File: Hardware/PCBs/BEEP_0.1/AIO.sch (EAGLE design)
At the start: 79 parts, among them IC1 ULN2803ASOP18, IC2 ULN2803ASOP18, IC3 74HC238SSOP, IC4 74HC238SSOP, IC5 TS34119SMD, U2 TB6612FNG, U3 ATXMEGA64D3-AU, X10 MICROMATCH-10, X3 MICROMATCH-8, X4 MICROMATCH-8, X5 MICROMATCH-8, X8 MICROMATCH-8, X9 MICROMATCH-4

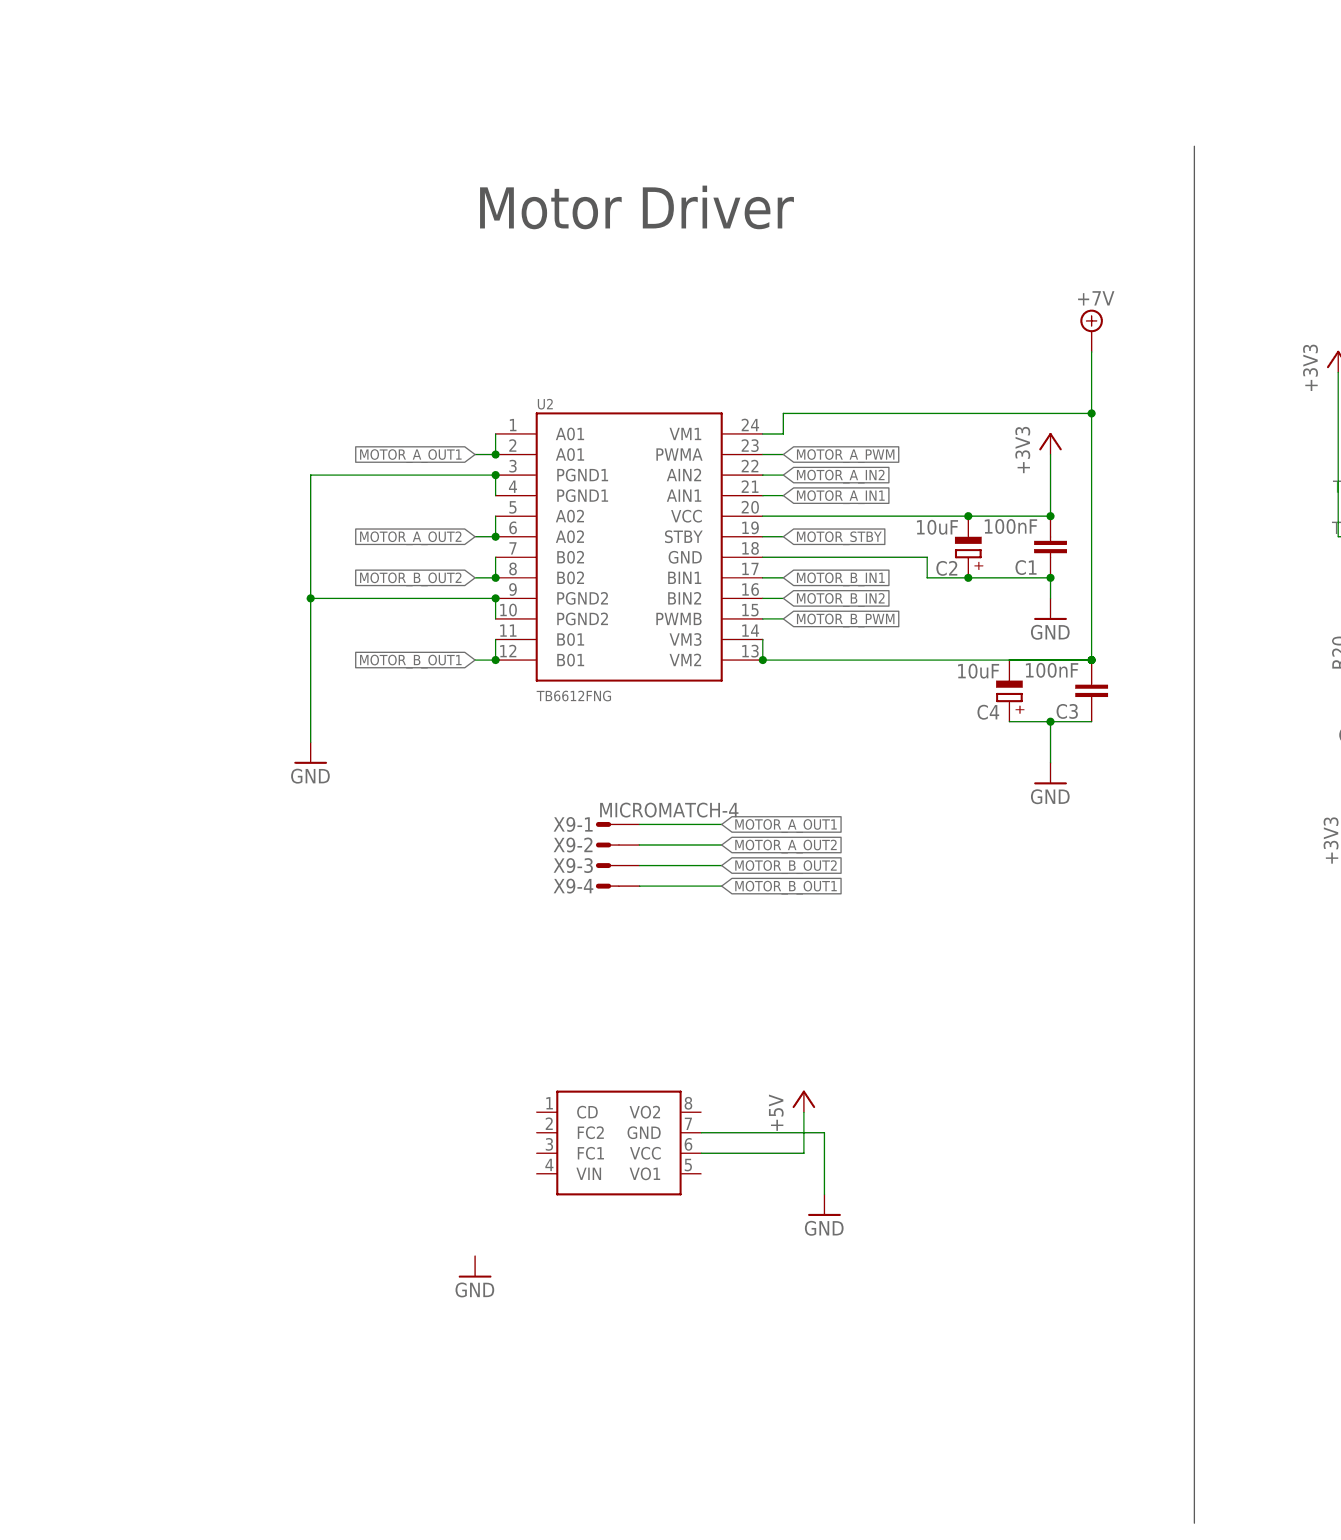
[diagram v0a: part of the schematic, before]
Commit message: routing
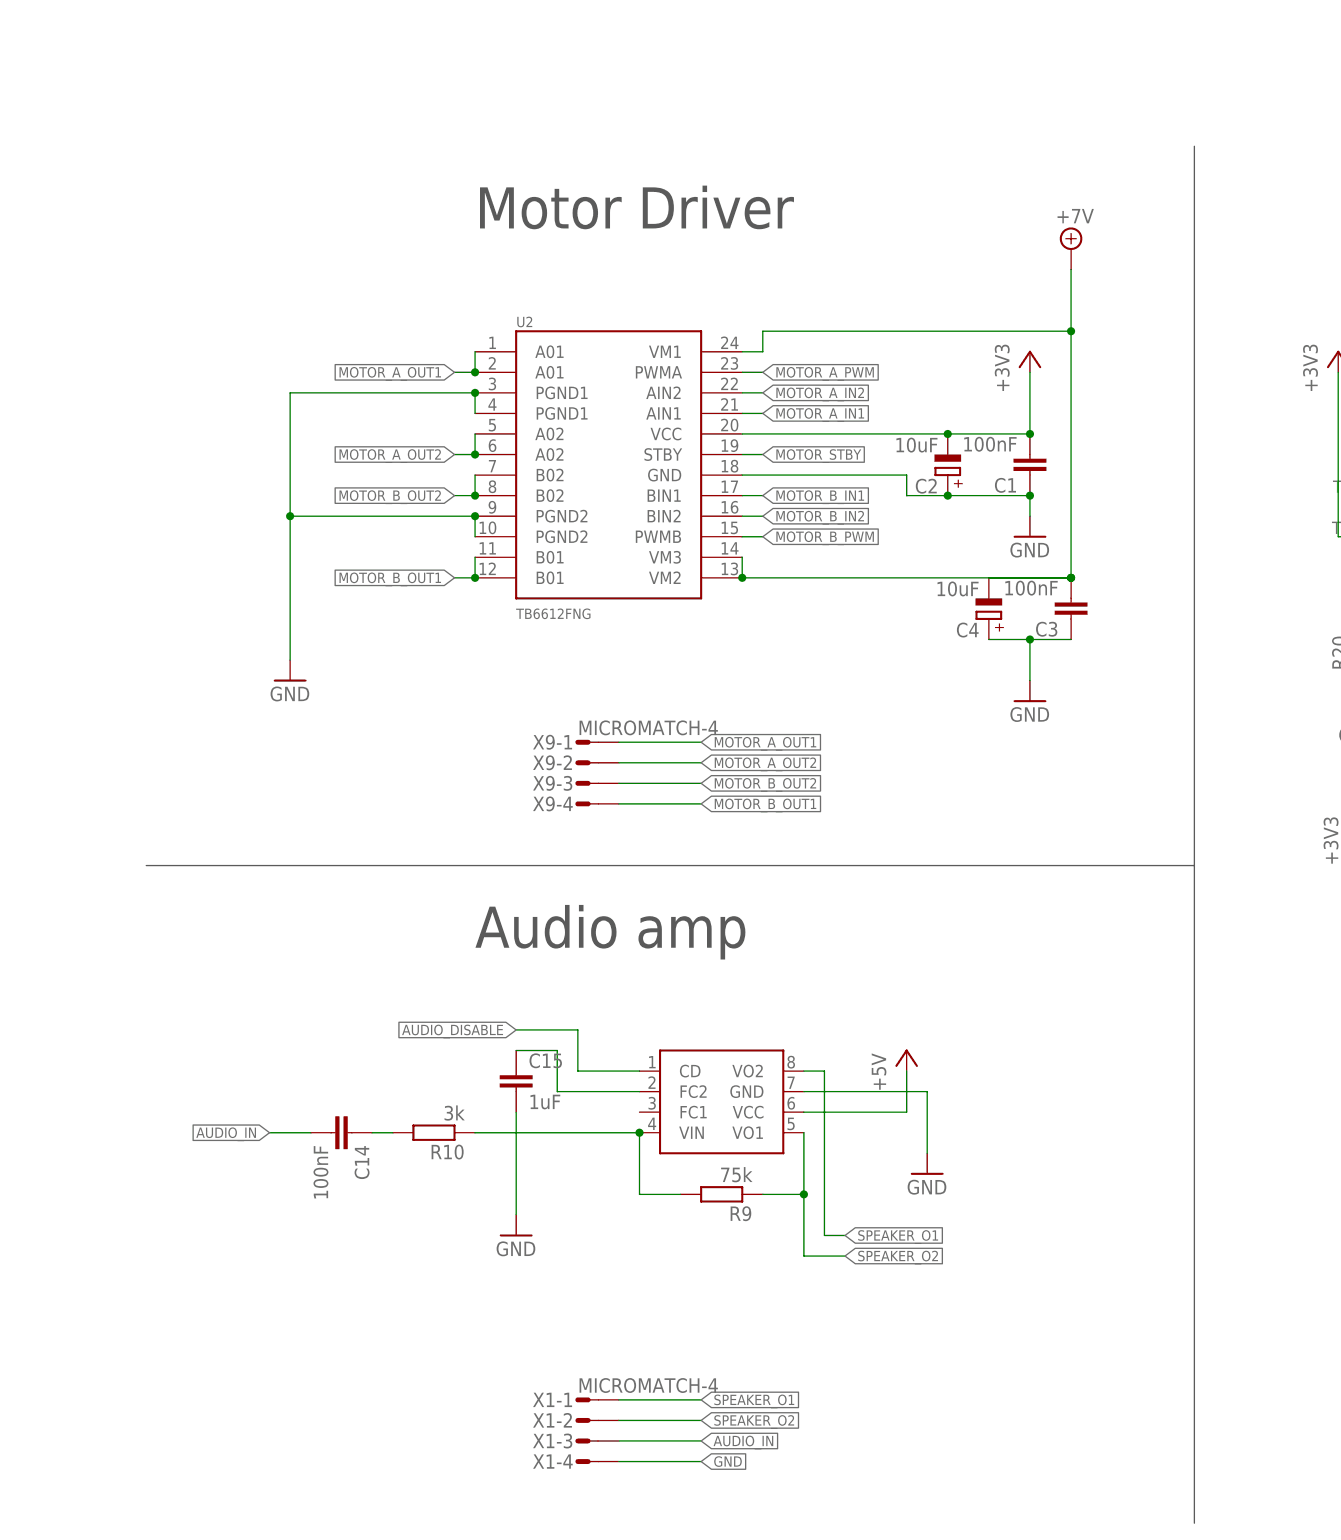
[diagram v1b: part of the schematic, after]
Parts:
- added C14: 100nF, rcl:C-EUC0603
- added C15: 1uF, rcl:C-EUC0603
- added R10: 3k, rcl:R-EU_R0603
- added R9: 75k, rcl:R-EU_R0603
- added X1: MICROMATCH-4, Con-amp-micromatch:MICROMATCH-4
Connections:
- new net AUDIO_DISABLE: IC5.CD
- new net AUDIO_IN: C14.2, X1-3.S
- new net N$15: IC5.VIN, R10.1, R9.2
- new net N$17: C14.1, R10.2
- new net N$36: C15.1, IC5.FC2
- new net SPEAKER_O1: IC5.VO2, X1-1.S
- new net SPEAKER_O2: IC5.VO1, R9.1, X1-2.S
- net GND: now also C15.2, X1-4.S
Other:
- note added: "Audio amp"
- moved on the sheet: C1, C2, C3, C4, U2, X9-1, X9-2, X9-3, X9-4
